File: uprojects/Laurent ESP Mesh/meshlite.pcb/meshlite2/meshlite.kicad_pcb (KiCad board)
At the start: 2 copper layers, 109.5 x 57.1 mm, 16 parts, among them J1 DCJ200-10-A-XX-K_REVA, J3 B5PS-VH, K2 FINDER-36.11, Q1 MMBT2222A, U1 MOUDLE-SEEEDUINO-XIAO-ESP32C3, U2 INA219, U3 YAAJ_DCDC_StepDown_LM2596

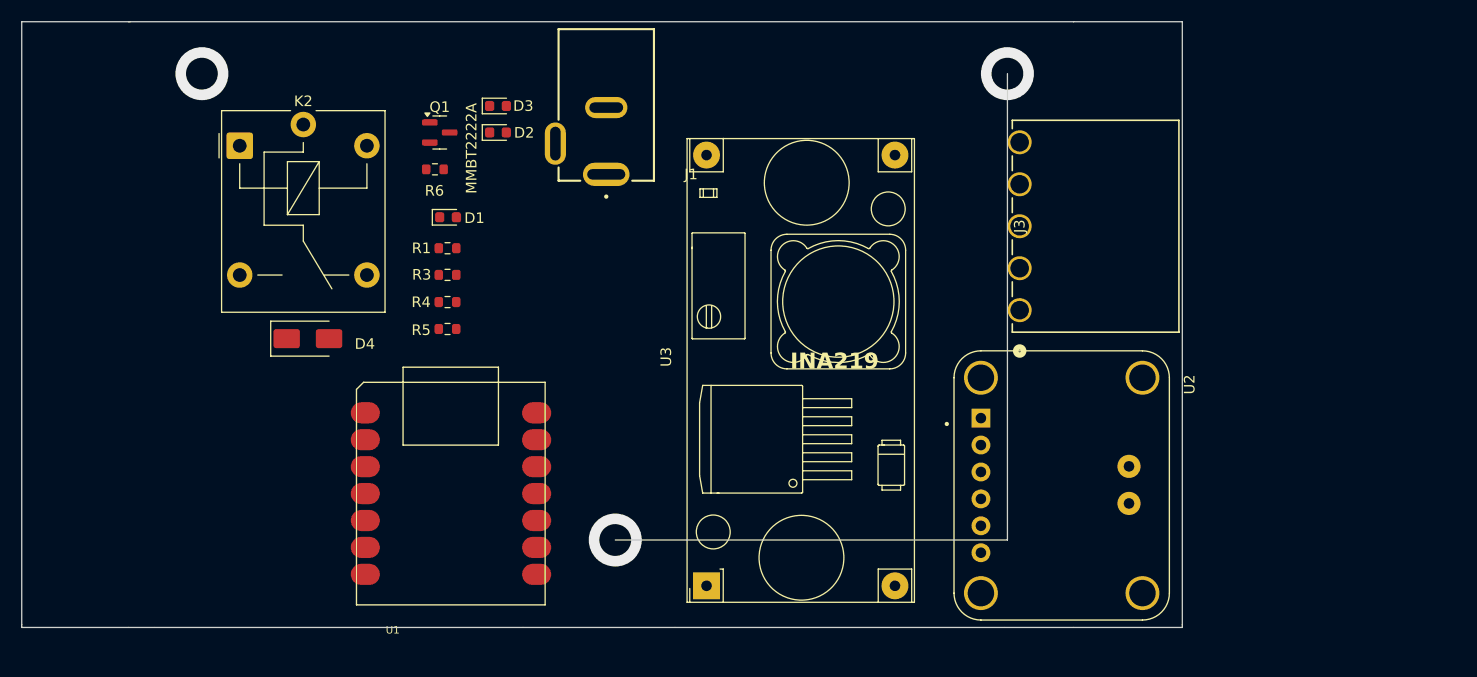
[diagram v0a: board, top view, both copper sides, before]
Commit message: Update 20 Feb 2026
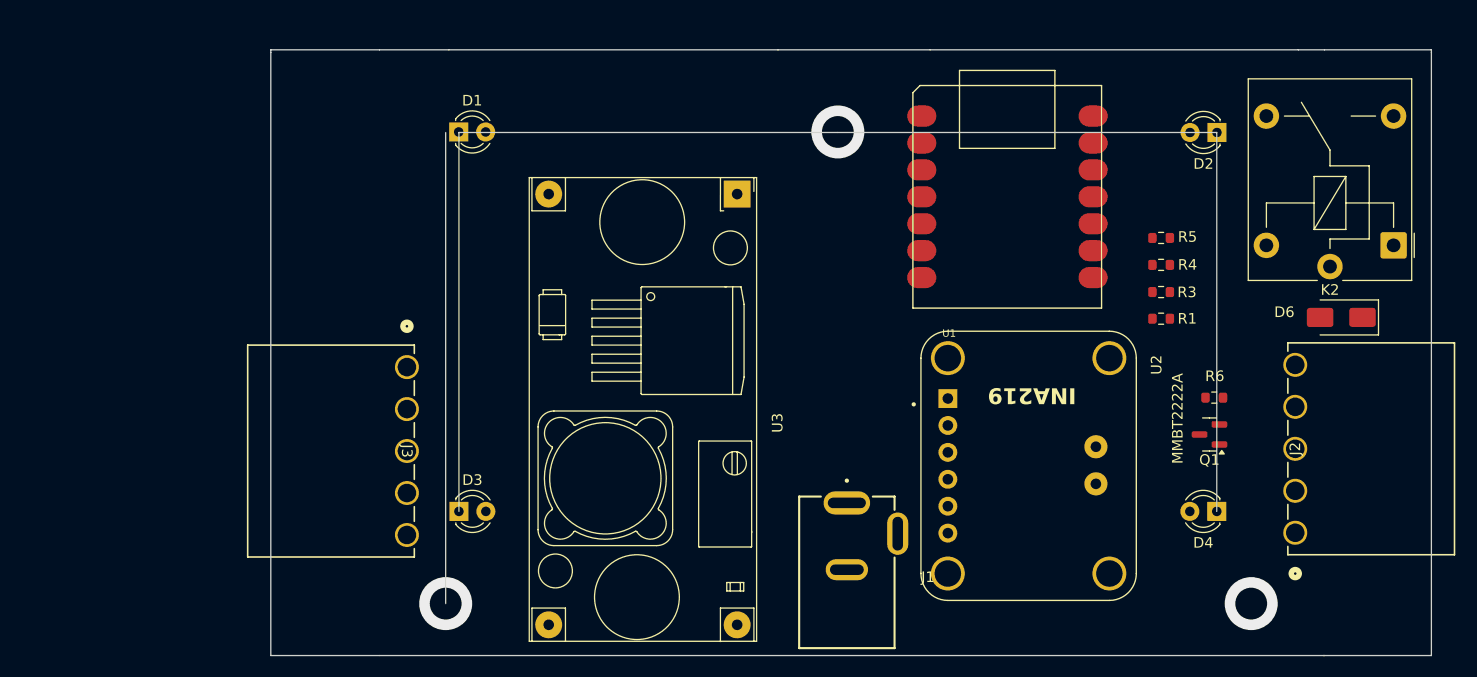
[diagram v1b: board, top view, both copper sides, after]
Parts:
- added D4: LED, LED_THT:LED_D3.0mm, F.Cu at (195.2, 84.3)
- added J2: B5PS-VH, footprints:CONN_B5PS-VH_JST, F.Cu at (202.7, 86.3)
- D1, D2, D3: footprint LED_SMD:LED_0603_1608Metric -> LED_THT:LED_D3.0mm
- moved K2 109.3 mm to (211.9, 59.2), turned to 180 degrees
- moved D6 97.5 mm to (207.0, 66.0), turned to 180 degrees
- moved Q1 78.0 mm to (194.6, 77.0), turned to 180 degrees
- moved R6 76.6 mm to (195.0, 73.6), turned to 180 degrees
- moved R5 67.9 mm to (190.0, 58.5), turned to 180 degrees
- moved D2 67.8 mm to (195.3, 48.5), turned to 180 degrees
- moved R1 67.7 mm to (190.0, 66.1), turned to 180 degrees
- moved R4 67.4 mm to (190.0, 61.0), turned to 180 degrees
- moved R3 67.3 mm to (190.0, 63.6), turned to 0 degrees
- moved U1 59.5 mm to (166.6, 65.1)
- moved J3 58.1 mm to (118.8, 70.7), turned to -90 degrees
- moved J1 49.6 mm to (160.3, 90.0), turned to 0 degrees
- moved D3 38.4 mm to (123.8, 84.3)
- moved U3 37.1 mm to (150.0, 54.4), turned to -90 degrees
- moved D1 8.11 mm to (123.7, 48.5)
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- renumbered D4 to D6
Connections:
- J3 pad 1: unconnected-(J3-Pad1) -> /24VDC-IN
- J3 pad 2: unconnected-(J3-Pad2) -> GND
- J3 pad 3: unconnected-(J3-Pad3) -> /PGND
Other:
- board size 109.5 x 57.1 mm -> 109.5 x 57.2 mm
